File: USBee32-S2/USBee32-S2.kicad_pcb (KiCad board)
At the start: 4 copper layers, 27.9 x 68.4 mm, 52 parts, among them IC1 IP4220CZ6, J1 USB_A, J2 TYPE-C-31-M-12, J3 Conn_01x18_Male, J4 S2B-PH-SM4-TB(LF)(SN), J5 Conn_01x22_Male, SW1 SW_Push, SW2 SW_Push, U1 ESP32-S2-WROOM-ESP32-S2-WROOM, U2 MMBT8050, U3 MMBT8050, U4 MCP73831-2-OT, U5 AMS1117-3.3, U6 CH340C

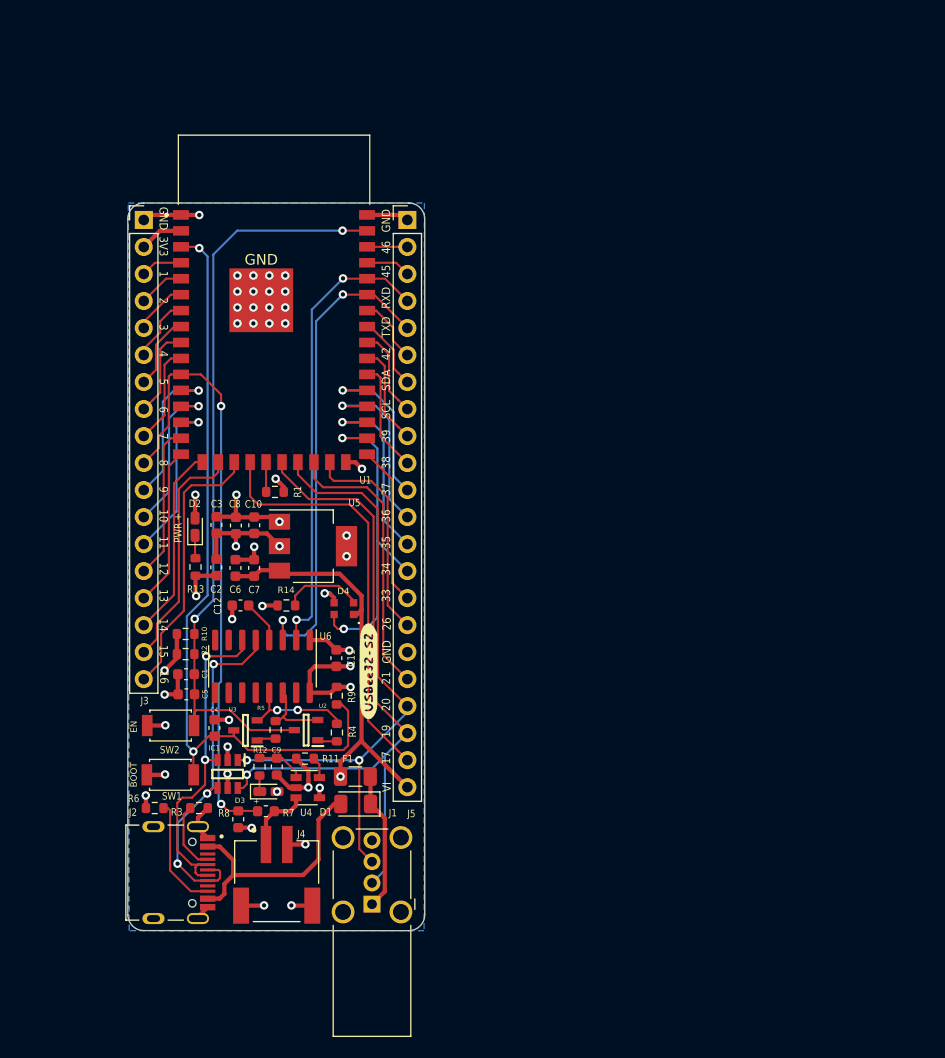
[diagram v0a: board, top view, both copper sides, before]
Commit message: Rotated board
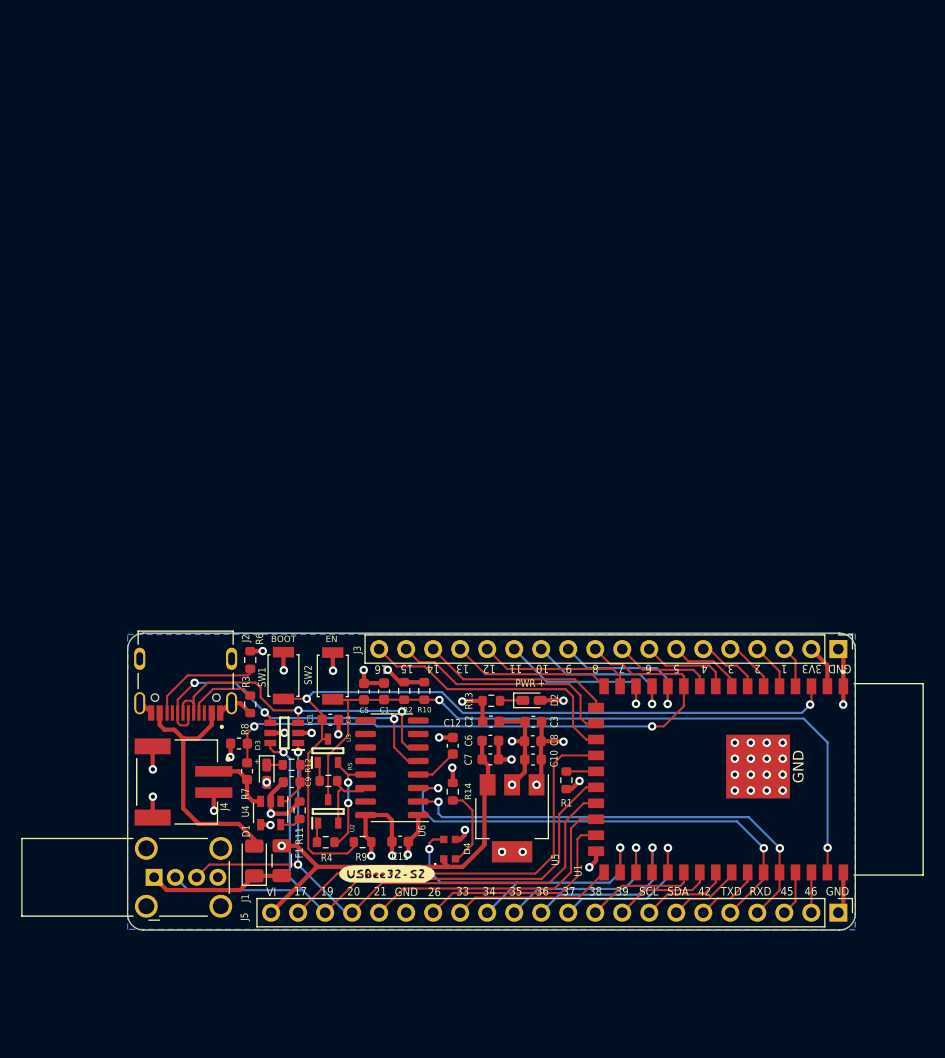
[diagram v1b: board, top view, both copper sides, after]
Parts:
- moved J3 76.8 mm to (203.8, 109.0), turned to 270 degrees
- moved J5 76.7 mm to (203.8, 133.8), turned to 270 degrees
- moved REF** 72.7 mm to (201.9, 114.8), turned to 90 degrees
- moved REF** 72.5 mm to (202.1, 124.1), turned to 90 degrees
- moved U1 64.1 mm to (196.2, 121.3), turned to 270 degrees
- moved GND 64.1 mm to (196.2, 120.1), turned to 270 degrees
- moved G1 55.3 mm to (190.1, 121.5), turned to 90 degrees
- moved G*** 46.9 mm to (184.1, 121.5), turned to 90 degrees
- moved R1 38.6 mm to (178.2, 121.4), turned to 90 degrees
- moved D2 35.6 mm to (174.9, 113.9), turned to 0 degrees
- moved C3 35.1 mm to (175.1, 115.9), turned to 0 degrees
- moved C8 34.5 mm to (175.0, 117.7), turned to 180 degrees
- moved C10 34.2 mm to (175.1, 119.4), turned to 180 degrees
- moved U5 31.7 mm to (173.1, 124.9), turned to 270 degrees
- moved R13 30.5 mm to (171.1, 113.9), turned to 180 degrees
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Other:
- board size 27.9 x 68.4 mm -> 68.4 x 27.9 mm

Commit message: Made suggested changes in schematics
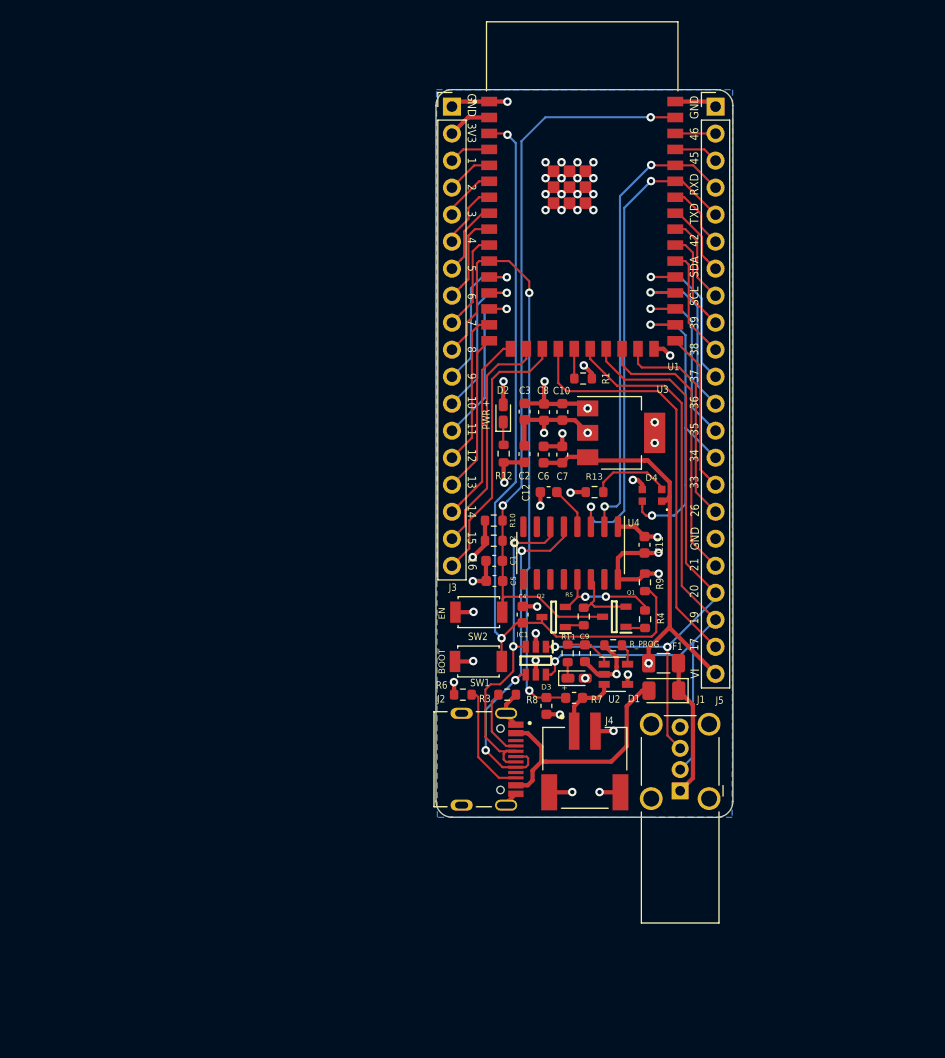
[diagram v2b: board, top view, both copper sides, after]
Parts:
- removed G***: LOGO, USBee32-S2-Label:usbee32s2-qr
- removed G***: LOGO, USBee32-S2-Label:usbee32s2-fs
- removed G***: LOGO, USBee32-S2-Label:largelabel
- removed G1: LOGO, WS2018:sralogo
- removed GND: SolderWirePad_1x01_SMD_5x10mm, Connector_Wire:SolderWirePad_1x01_SMD_5x10mm
- removed the R11 at (153.1, 124.2)
- removed REF**: OSHW-Logo_5.7x6mm_SilkScreen, Designs:OSHW-Logo_5.7x6mm_SilkScreen
- removed REF**: KiCad-Logo_5mm_SilkScreen, Designs:KiCad-Logo_5mm_SilkScreen
- added R_PROG: 4.7k, Resistor_SMD:R_0603_1608Metric, F.Cu at (182.6, 108.7)
- moved J5 76.7 mm to (192.2, 58.0), turned to 0 degrees
- moved J3 62.6 mm to (167.4, 58.0), turned to 0 degrees
- moved U1 58.1 mm to (179.7, 65.5), turned to 0 degrees
- moved J1 50.1 mm to (188.9, 122.4), turned to 90 degrees
- moved D1 41.7 mm to (187.4, 112.9), turned to 180 degrees
- moved F1 40.4 mm to (187.3, 110.4), turned to 0 degrees
- moved D4 38.3 mm to (186.2, 94.6), turned to 0 degrees
- moved R1 37.8 mm to (179.8, 83.6), turned to 180 degrees
- moved U3 37.7 mm to (183.3, 88.7), turned to 0 degrees
- moved R4 36.6 mm to (185.6, 106.2), turned to 270 degrees
- moved C11 36.2 mm to (185.5, 99.2), turned to 90 degrees
- moved R9 36.1 mm to (185.6, 102.8), turned to 90 degrees
- moved J4 35.2 mm to (179.9, 116.7), turned to 0 degrees
- moved U2 35.0 mm to (182.8, 111.4), turned to 0 degrees
- moved C10 32.8 mm to (177.8, 86.7), turned to 270 degrees
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- renumbered U2 to Q1, U3 to Q2, R12 to R11, R13 to R12, R14 to R13, U4 to U2, U5 to U3, U6 to U4
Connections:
- net /GPIO0 renamed /GPIO_0
- net /GPIO1 renamed /GPIO_1
- net /GPIO10 renamed /GPIO_10
- net /GPIO11 renamed /GPIO_11
- net /GPIO12 renamed /GPIO_12
- net /GPIO13 renamed /GPIO_13
- net /GPIO14 renamed /GPIO_14
- net /GPIO15 renamed /GPIO_15
- net /GPIO16 renamed /GPIO_16
- net /GPIO17 renamed /GPIO_17
- net /GPIO18 renamed /GPIO_18
- net /GPIO19 renamed /GPIO_19
- net /GPIO2 renamed /GPIO_2
- net /GPIO20 renamed /GPIO_20
- net /GPIO21 renamed /GPIO_21
- net /GPIO26 renamed /GPIO_26
- net /GPIO3 renamed /GPIO_3
- net /GPIO33 renamed /GPIO_33
- net /GPIO34 renamed /GPIO_34
- net /GPIO35 renamed /GPIO_35
- net /GPIO36 renamed /GPIO_36
- net /GPIO37 renamed /GPIO_37
- net /GPIO38 renamed /GPIO_38
- net /GPIO39 renamed /GPIO_39
- net /GPIO4 renamed /GPIO_4
- net /GPIO40 renamed /GPIO_40
- net /GPIO41 renamed /GPIO_41
- net /GPIO42 renamed /GPIO_42
- net /GPIO45 renamed /GPIO_45
- net /GPIO46 renamed /GPIO_46
- net /GPIO5 renamed /GPIO_5
- net /GPIO6 renamed /GPIO_6
- net /GPIO7 renamed /GPIO_7
- net /GPIO8 renamed /GPIO_8
- net /GPIO9 renamed /GPIO_9
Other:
- board size 68.4 x 27.9 mm -> 27.9 x 68.4 mm
